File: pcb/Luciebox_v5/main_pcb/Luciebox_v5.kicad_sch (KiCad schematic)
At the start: 64 parts, among them J1 USB_B_Mini, J2 USB_B_Mini, Q1 P-Channel MOSFET, Q2 NPN transistor, T1 terminal_8x1, T2 terminal_3x1, T4 terminal_8x1, T5 terminal_3x1, T6 terminal_8x1, T7 terminal_8x1, T8 terminal_8x1, U1 CA56-12SRWA, U2 8X8PADS, U3 ATmega328-PU, Y1 16MHz

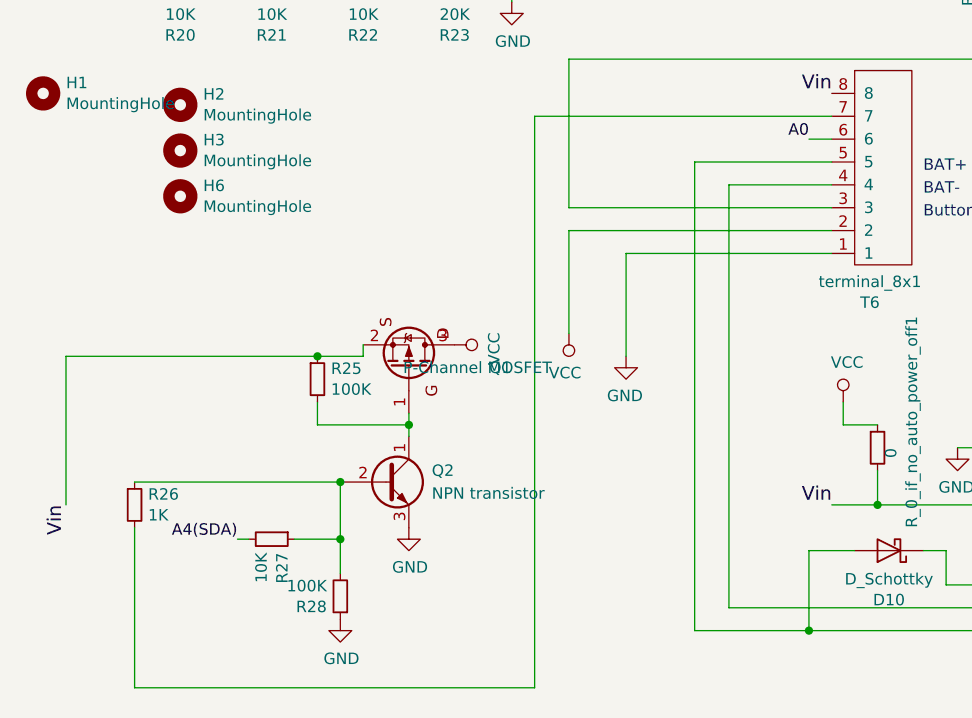
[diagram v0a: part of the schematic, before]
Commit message: Pcb V5
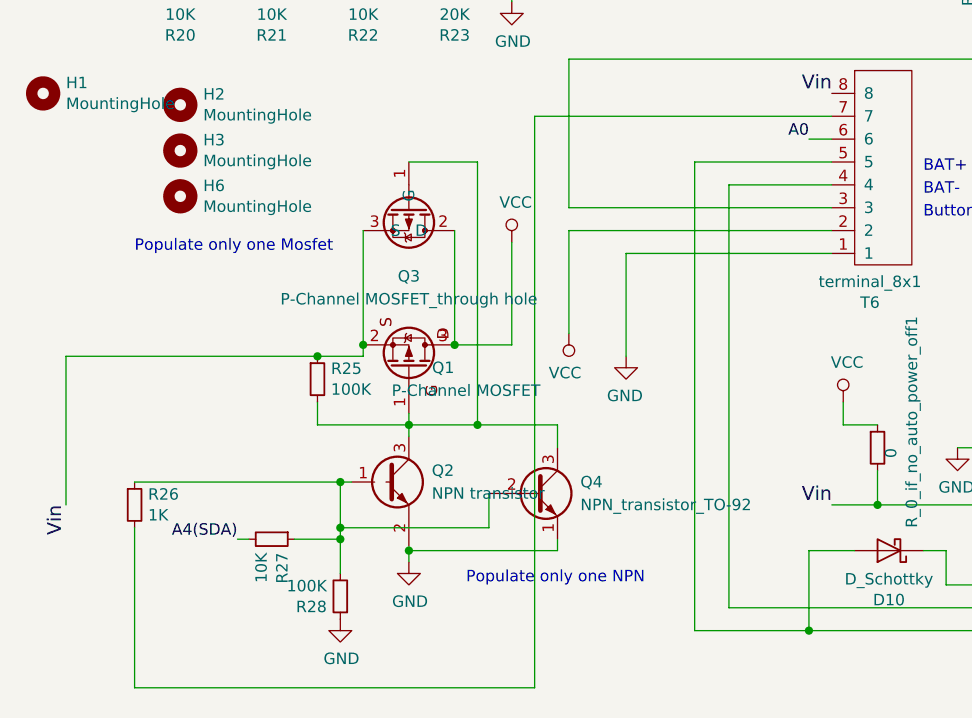
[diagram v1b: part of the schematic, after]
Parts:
- added Q3: P-Channel MOSFET_through hole, Package_TO_SOT_THT:TO-218-3_Vertical, symbol Luciebox_components:P-Channel MOSFET_through hole
- added Q4: NPN_transistor_TO-92, Package_TO_SOT_THT:TO-92, symbol Luciebox_components:NPN_transistor_TO-92
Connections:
- net GND: now also Q2.2 (B), Q4.1 (C); no longer Q2.3 (E)
- net VCC: now also Q3.2 (D)
- net Vin: now also Q3.3 (S)
- net at R26.1, R27.1, R28.2: now also Q2.1 (C), Q4.2 (B); no longer Q2.2 (B)
- net at Q1.1 (G), R25.2: now also Q2.3 (E), Q3.1 (G), Q4.3 (E); no longer Q2.1 (C)
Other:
- note added: "Populate only one Mosfet"
- note added: "Populate only one NPN"
- moved on the sheet: Q2
